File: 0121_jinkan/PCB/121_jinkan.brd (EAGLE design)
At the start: 25.4 x 33 mm, 12 parts

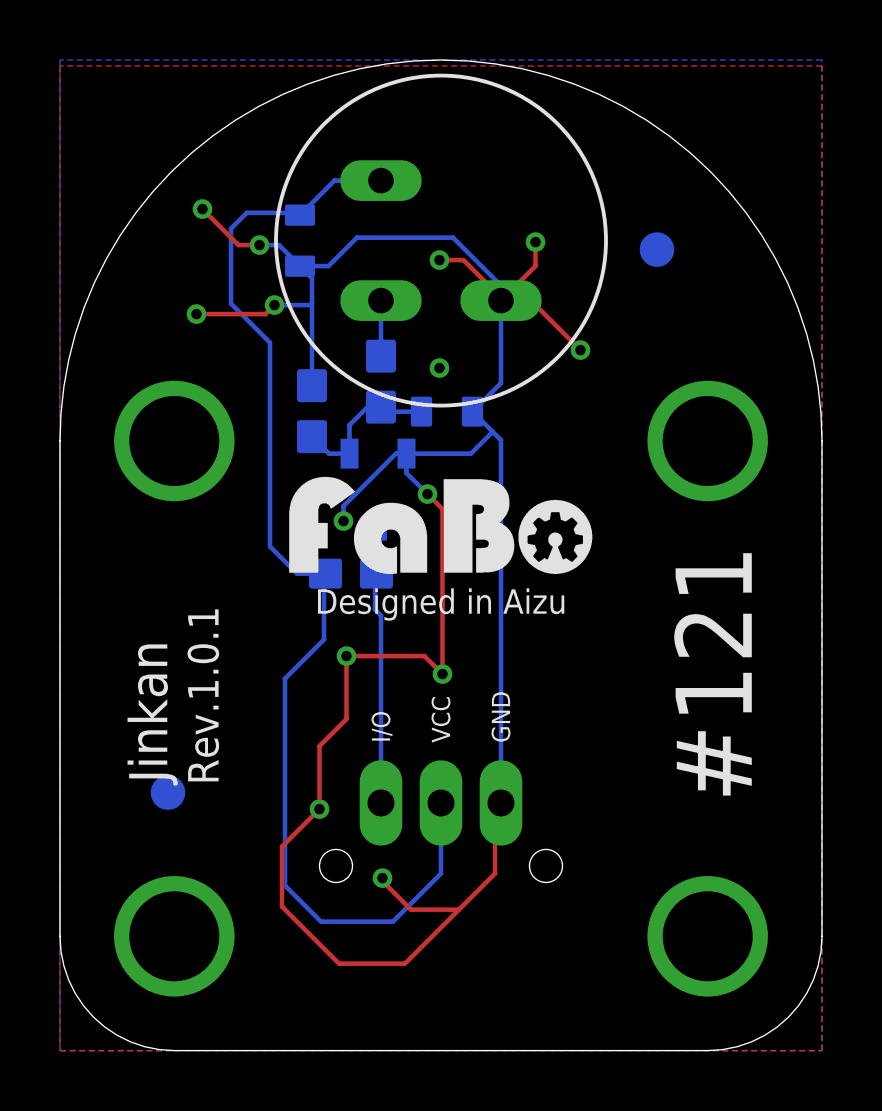
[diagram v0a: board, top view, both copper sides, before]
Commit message: 121_jinkan　ロゴ修正、リファイン
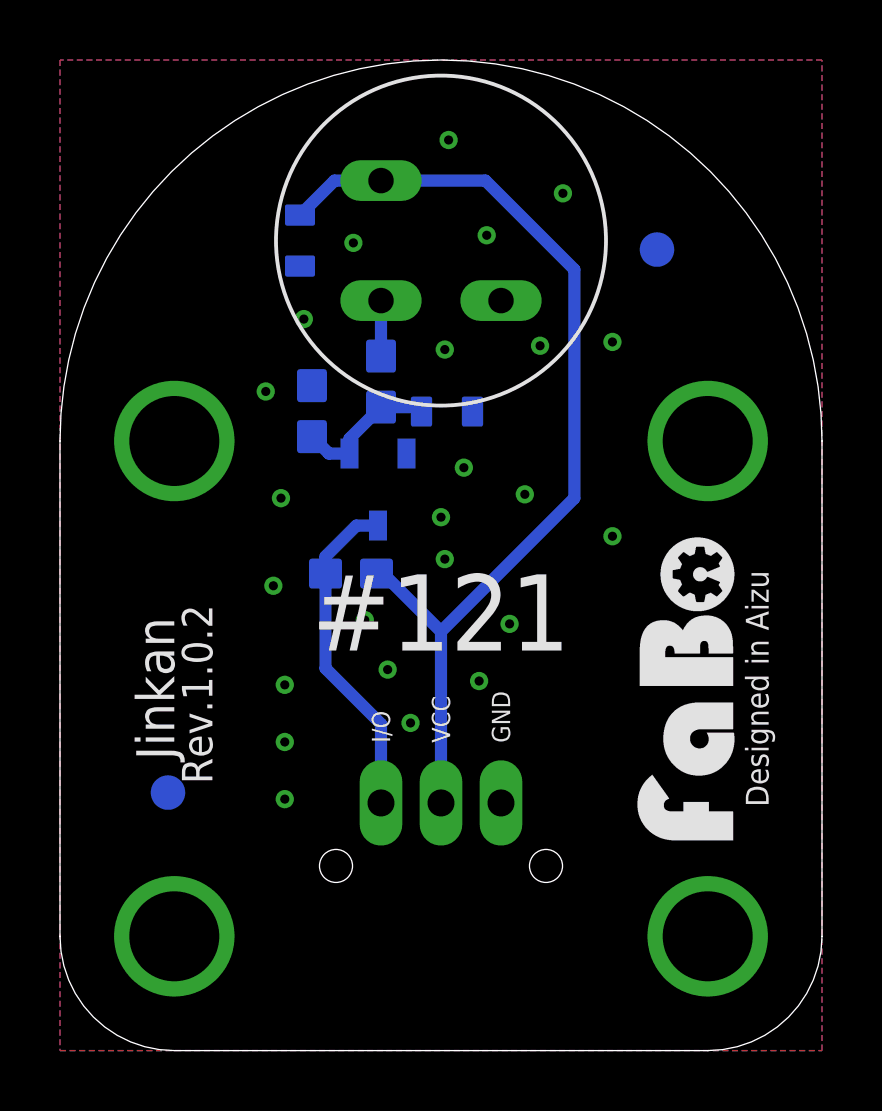
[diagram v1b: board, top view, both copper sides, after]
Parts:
- removed U$3: (no value), FaBo-etc:LOGO_FABO_MS_BOTTOM
- added LOGO1: (no value), component:LOGO_FABO_M
- turned R3 to 180 degrees
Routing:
- net GND: track 88.1 -> 0.00 mm, vias 14 -> 24
- net VCC: track 38.8 -> 33.4 mm
- net I/O: track 9.37 -> 11.2 mm
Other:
- board text added: "Rev.1.0.2"
- board text removed: "Rev.1.0.1"
